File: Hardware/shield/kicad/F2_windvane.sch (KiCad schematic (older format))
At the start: 7 parts, among them U1 MCP6244

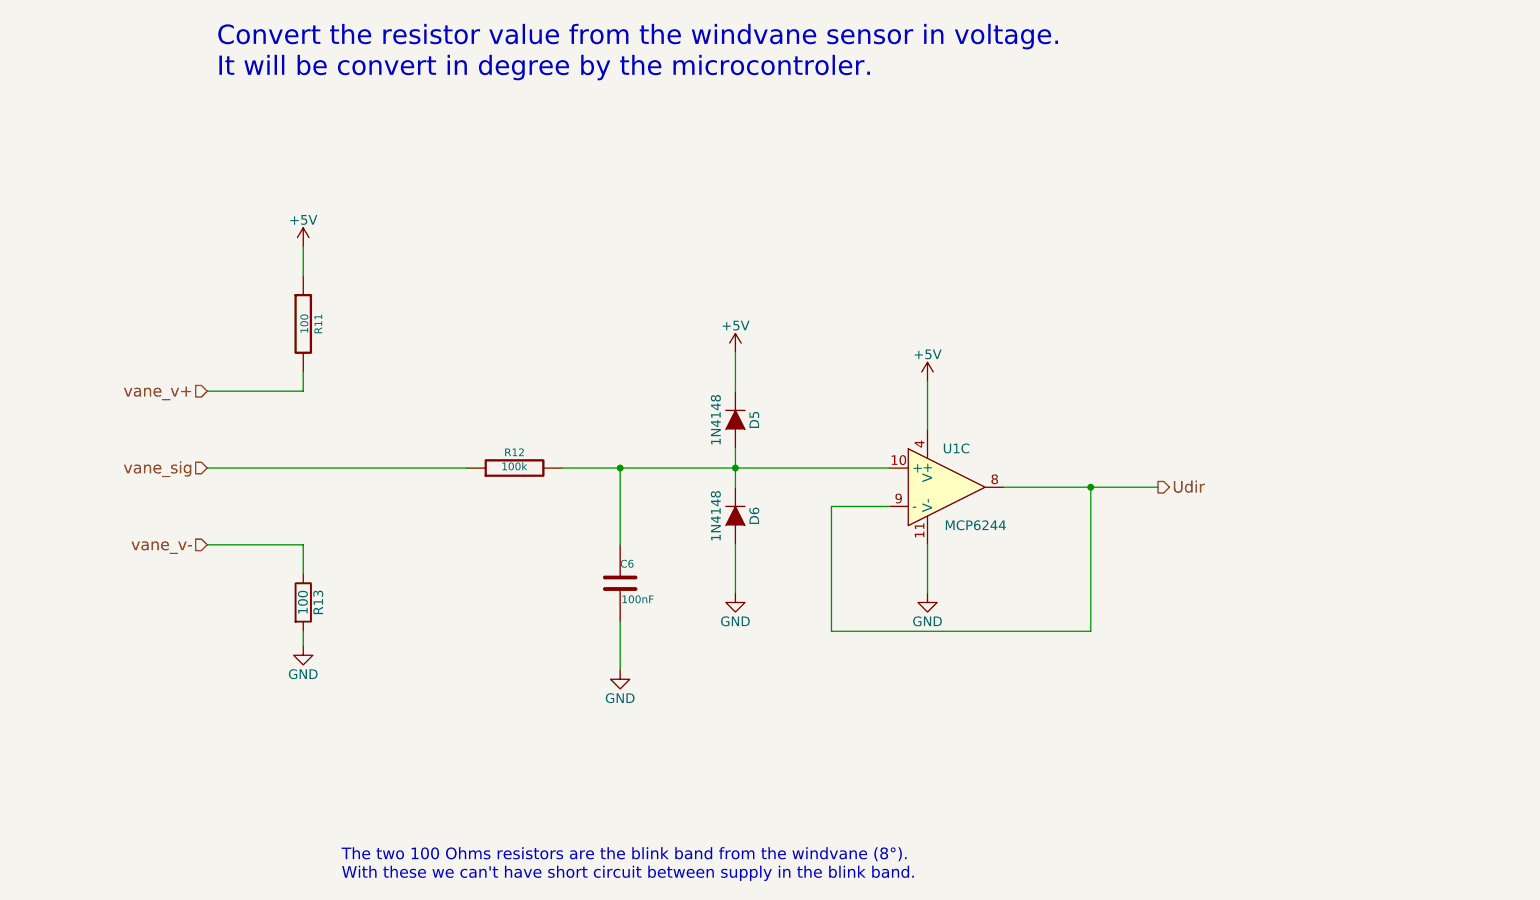
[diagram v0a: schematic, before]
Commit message: move to digital 1.1.1
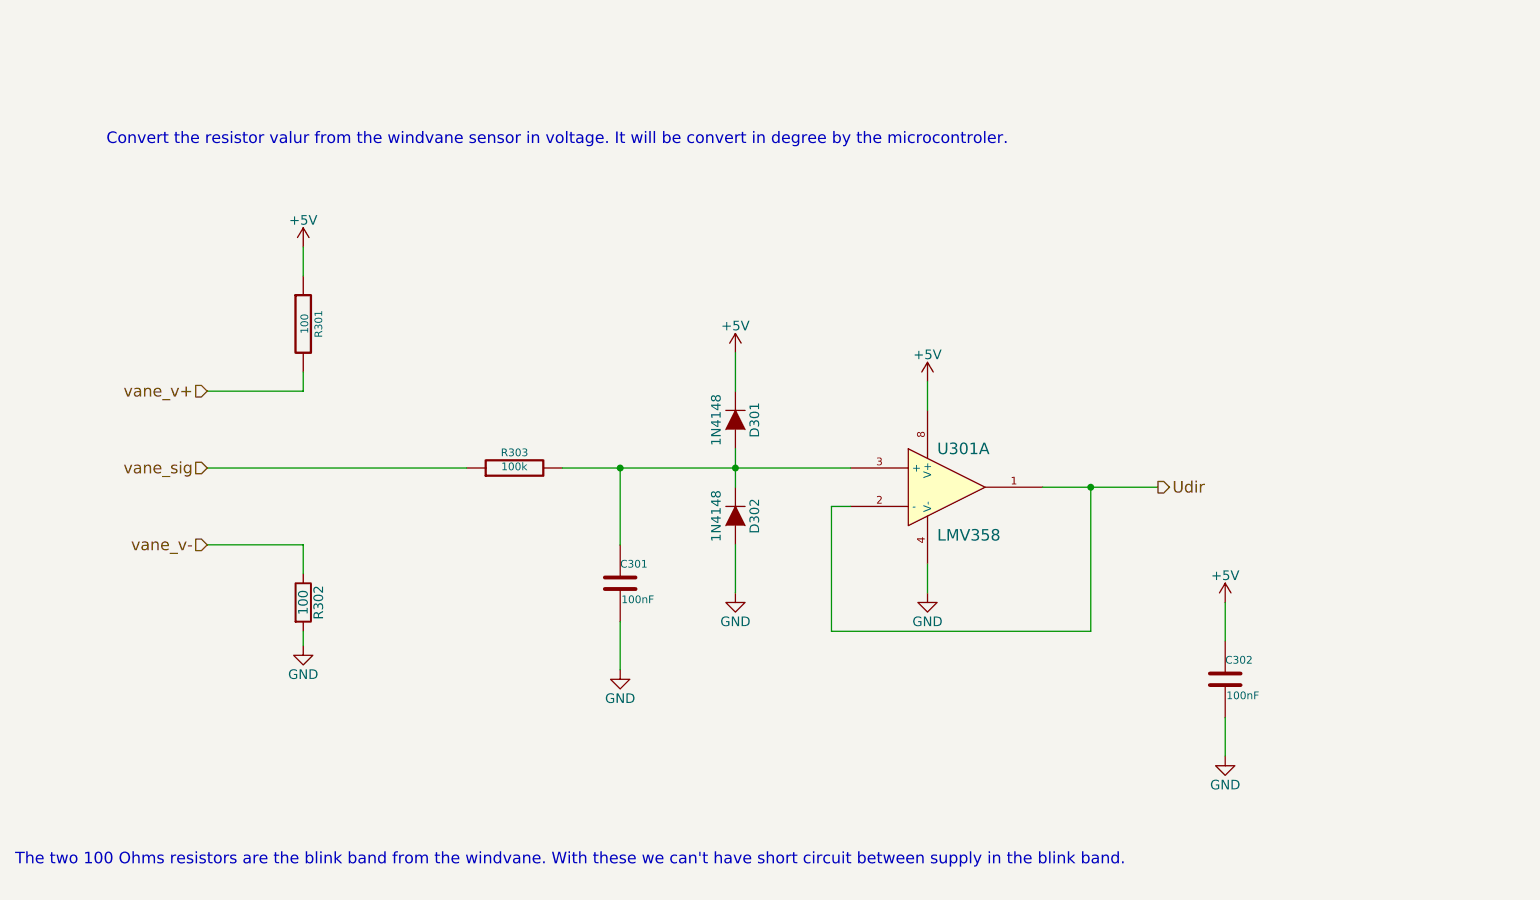
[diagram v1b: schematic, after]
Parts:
- removed U1: MCP6244, Housings_DIP:DIP-14_W7.62mm_LongPads, symbol MCP6004
- added C302: 100nF, Capacitors_ThroughHole:C_Rect_L7_W2.5_P5, symbol C-RESCUE-Windlogger
- added U301: LMV358, Housings_DIP:DIP-8_W7.62mm_LongPads, symbol LM358-RESCUE-Windlogger
- D301: renamed from D5; footprint Discret:DO-35 -> Diodes_ThroughHole:Diode_DO-35_SOD27_Horizontal_RM10
- D302: renamed from D6; footprint Discret:DO-35 -> Diodes_ThroughHole:Diode_DO-35_SOD27_Horizontal_RM10
- R301: renamed from R11; footprint Discret:R3-LARGE_PADS -> Discret:R4
- R302: renamed from R13; footprint Discret:R3-LARGE_PADS -> Discret:R4
- R303: renamed from R12; footprint Discret:R3-LARGE_PADS -> Discret:R4
- renumbered C6 to C301
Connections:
- net +5V: now also C302.1, U301.8 (V+)
- net GND: now also C302.2, U301.4 (V-)
- net Udir: now also U301.1, U301.2 (-)
- net at C301.1, D301.2 (A), D302.1 (K)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: now also U301.3 (+)
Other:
- note added: "Convert the resistor valur from the windvane sensor in voltage. It will be convert in degree by the microcontroler."
- note added: "The two 100 Ohms resistors are the blink band from the windvane. With these we can't have short circuit between supply in the blink band."
- note removed: "Convert the resistor value from the windvane sensor in voltage. \nIt will be convert in degree by the microcontroler."
- note removed: "The two 100 Ohms resistors are the blink band from the windvane (8°).\nWith these we can't have short circuit between supply in the blink band."
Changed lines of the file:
@@
 $Descr A4 11693 8268
 encoding utf-8
-Sheet 3 5
+Sheet 3 6
 Title "Windvane function"
 Date "2016-10-16"
@@
 $EndDescr
 $Comp
-L R-RESCUE-Windlogger R11
+L R-RESCUE-Windlogger R301
 U 1 1 561261A3
 P 4050 2550
-F 0 "R11" V 4130 2550 40  0000 C CNN
+F 0 "R301" V 4130 2550 40  0000 C CNN
 F 1 "100" V 4057 2551 40  0000 C CNN
-F 2 "Discret:R3-LARGE_PADS" V 3980 2550 30  0001 C CNN
+F 2 "Discret:R4" V 3980 2550 30  0001 C CNN
 F 3 "~" H 4050 2550 30  0000 C CNN
 F 4 "0.125W" V 4050 2550 60  0001 C CNN "Puissance"
@@
 $EndComp
 $Comp
-L C-RESCUE-Windlogger C6
+L C-RESCUE-Windlogger C301
 U 1 1 561264FC
 P 5700 3900
-F 0 "C6" H 5700 4000 40  0000 L CNN
+F 0 "C301" H 5700 4000 40  0000 L CNN
 F 1 "100nF" H 5706 3815 40  0000 L CNN
 F 2 "Capacitors_ThroughHole:C_Rect_L7_W2.5_P5" H 5738 3750 30  0001 C CNN
@@
 	4050 2150 4050 2300
 Wire Wire Line
-	7700 3400 8500 3400
+	7900 3400 8500 3400
 Wire Wire Line
 	5700 3300 5700 3700
@@
 	5700 4350 5700 4100
 Wire Wire Line
-	7300 2850 7300 3100
-Wire Wire Line
-	7300 3700 7300 3950
+	7300 3000 7300 2850
+Wire Wire Line
+	7300 3800 7300 3950
 Text HLabel 8500 3400 2    60   Output ~ 0
 Udir
@@
 vane_sig
 $Comp
-L R-RESCUE-Windlogger R12
+L C-RESCUE-Windlogger C302
+U 1 1 56126B37
+P 8850 4400
+F 0 "C302" H 8850 4500 40  0000 L CNN
+F 1 "100nF" H 8856 4315 40  0000 L CNN
+F 2 "Capacitors_ThroughHole:C_Rect_L7_W2.5_P5" H 8888 4250 30  0001 C CNN
+F 3 "~" H 8850 4400 60  0000 C CNN
+F 4 "25V" H 8850 4400 60  0001 C CNN "Tension"
+	1    8850 4400
+	1    0    0    -1
+$EndComp
+Wire Wire Line
+	8850 4000 8850 4200
+Wire Wire Line
+	8850 4600 8850 4800
+$Comp
+L R-RESCUE-Windlogger R303
 U 1 1 5612799B
 P 5150 3300
-F 0 "R12" V 5230 3300 40  0000 C CNN
+F 0 "R303" V 5230 3300 40  0000 C CNN
 F 1 "100k" V 5157 3301 40  0000 C CNN
-F 2 "Discret:R3-LARGE_PADS" V 5080 3300 30  0001 C CNN
+F 2 "Discret:R4" V 5080 3300 30  0001 C CNN
 F 3 "~" H 5150 3300 30  0000 C CNN
 F 4 "0.125W" V 5150 3300 60  0001 C CNN "Puissance"
@@
 	3550 3300 4900 3300
 Wire Wire Line
-	5400 3300 7100 3300
+	5400 3300 6900 3300
 Wire Wire Line
 	8150 4150 8150 3400
@@
 vane_v-
 Wire Wire Line
-	6800 3500 7100 3500
+	6900 3500 6800 3500
 Wire Wire Line
 	6800 3500 6800 4150
@@
 	6300 3700 6300 3950
 $Comp
-L +5V #PWR034
+L LM358-RESCUE-Windlogger U301
+U 1 1 561263BB
+P 7400 3400
+F 0 "U301" H 7350 3600 60  0000 L CNN
+F 1 "LMV358" H 7350 3150 60  0000 L CNN
+F 2 "Housings_DIP:DIP-8_W7.62mm_LongPads" H 7400 3400 60  0001 C CNN
+F 3 "" H 7400 3400 60  0000 C CNN
+	1    7400 3400
+	1    0    0    -1
+$EndComp
+$Comp
+L +5V #PWR031
 U 1 1 573BED92
 P 7300 2850
-F 0 "#PWR034" H 7300 2700 50  0001 C CNN
+F 0 "#PWR031" H 7300 2700 50  0001 C CNN
 F 1 "+5V" H 7300 2990 50  0000 C CNN
 F 2 "" H 7300 2850 50  0000 C CNN
@@
 $EndComp
 $Comp
-L +5V #PWR035
+L +5V #PWR032
+U 1 1 573BEDC7
+P 8850 4000
+F 0 "#PWR032" H 8850 3850 50  0001 C CNN
+F 1 "+5V" H 8850 4140 50  0000 C CNN
+F 2 "" H 8850 4000 50  0000 C CNN
+F 3 "" H 8850 4000 50  0000 C CNN
+	1    8850 4000
+	1    0    0    -1
+$EndComp
+$Comp
+L +5V #PWR033
 U 1 1 573D0C26
 P 4050 2150
-F 0 "#PWR035" H 4050 2000 50  0001 C CNN
+F 0 "#PWR033" H 4050 2000 50  0001 C CNN
 F 1 "+5V" H 4050 2290 50  0000 C CNN
 F 2 "" H 4050 2150 50  0000 C CNN
@@
 $EndComp
 $Comp
-L +5V #PWR036
+L +5V #PWR034
 U 1 1 573D0D74
 P 6300 2700
-F 0 "#PWR036" H 6300 2550 50  0001 C CNN
+F 0 "#PWR034" H 6300 2550 50  0001 C CNN
 F 1 "+5V" H 6300 2840 50  0000 C CNN
 F 2 "" H 6300 2700 50  0000 C CNN
@@
 $EndComp
 $Comp
-L R R13
+L R R302
 U 1 1 57E81F25
 P 4050 4000
-F 0 "R13" V 4130 4000 50  0000 C CNN
+F 0 "R302" V 4130 4000 50  0000 C CNN
 F 1 "100" V 4050 4000 50  0000 C CNN
-F 2 "Discret:R3-LARGE_PADS" V 3980 4000 50  0001 C CNN
+F 2 "Discret:R4" V 3980 4000 50  0001 C CNN
 F 3 "" H 4050 4000 50  0000 C CNN
 	1    4050 4000
@@
 Wire Wire Line
 	4050 4150 4050 4150
-Text Notes 3600 1275 0    100  ~ 0
-Convert the resistor value from the windvane sensor in voltage. \nIt will be convert in degree by the microcontroler.
-Text Notes 4250 5450 0    60   ~ 0
-The two 100 Ohms resistors are the blink band from the windvane (8°).\nWith these we can't have short circuit between supply in the blink band.
-$Comp
-L GND #PWR037
+Text Notes 3025 1625 0    60   ~ 0
+Convert the resistor valur from the windvane sensor in voltage. It will be convert in degree by the microcontroler.
+Text Notes 2550 5375 0    60   ~ 0
+The two 100 Ohms resistors are the blink band from the windvane. With these we can't have short circuit between supply in the blink band.
+$Comp
+L GND #PWR035
 U 1 1 58046061
 P 4050 4225
-F 0 "#PWR037" H 4050 3975 50  0001 C CNN
+F 0 "#PWR035" H 4050 3975 50  0001 C CNN
 F 1 "GND" H 4050 4075 50  0000 C CNN
 F 2 "" H 4050 4225 50  0000 C CNN
@@
 	4050 4225 4050 4150
 $Comp
-L GND #PWR038
+L GND #PWR036
 U 1 1 580460B8
 P 5700 4350
-F 0 "#PWR038" H 5700 4100 50  0001 C CNN
+F 0 "#PWR036" H 5700 4100 50  0001 C CNN
 F 1 "GND" H 5700 4200 50  0000 C CNN
 F 2 "" H 5700 4350 50  0000 C CNN
@@
 $EndComp
 $Comp
-L GND #PWR039
+L GND #PWR037
 U 1 1 580460EC
 P 6300 3950
-F 0 "#PWR039" H 6300 3700 50  0001 C CNN
+F 0 "#PWR037" H 6300 3700 50  0001 C CNN
 F 1 "GND" H 6300 3800 50  0000 C CNN
 F 2 "" H 6300 3950 50  0000 C CNN
@@
 $EndComp
 $Comp
-L GND #PWR040
+L GND #PWR038
 U 1 1 58046118
 P 7300 3950
-F 0 "#PWR040" H 7300 3700 50  0001 C CNN
+F 0 "#PWR038" H 7300 3700 50  0001 C CNN
 F 1 "GND" H 7300 3800 50  0000 C CNN
 F 2 "" H 7300 3950 50  0000 C CNN
@@
 $EndComp
 $Comp
-L D D5
+L GND #PWR039
+U 1 1 58046144
+P 8850 4800
+F 0 "#PWR039" H 8850 4550 50  0001 C CNN
+F 1 "GND" H 8850 4650 50  0000 C CNN
+F 2 "" H 8850 4800 50  0000 C CNN
+F 3 "" H 8850 4800 50  0000 C CNN
+	1    8850 4800
+	1    0    0    -1
+$EndComp
+$Comp
+L D D301
 U 1 1 580461AD
 P 6300 3050
-F 0 "D5" H 6300 3150 50  0000 C CNN
+F 0 "D301" H 6300 3150 50  0000 C CNN
 F 1 "1N4148" H 6300 2950 50  0000 C CNN
-F 2 "Discret:DO-35" H 6300 3050 50  0001 C CNN
+F 2 "Diodes_ThroughHole:Diode_DO-35_SOD27_Horizontal_RM10" H 6300 3050 50  0001 C CNN
 F 3 "" H 6300 3050 50  0000 C CNN
 	1    6300 3050
@@
 $EndComp
 $Comp
-L D D6
+L D D302
 U 1 1 58046207
 P 6300 3550
-F 0 "D6" H 6300 3650 50  0000 C CNN
+F 0 "D302" H 6300 3650 50  0000 C CNN
 F 1 "1N4148" H 6300 3450 50  0000 C CNN
-F 2 "Discret:DO-35" H 6300 3550 50  0001 C CNN
+F 2 "Diodes_ThroughHole:Diode_DO-35_SOD27_Horizontal_RM10" H 6300 3550 50  0001 C CNN
 F 3 "" H 6300 3550 50  0000 C CNN
 	1    6300 3550
 	0    1    1    0
 $EndComp
-$Comp
-L MCP6004 U1
-U 3 1 58593AA6
-P 7400 3400
-F 0 "U1" H 7450 3600 50  0000 C CNN
-F 1 "MCP6244" H 7550 3200 50  0000 C CNN
-F 2 "Housings_DIP:DIP-14_W7.62mm_LongPads" H 7350 3500 50  0001 C CNN
-F 3 "" H 7450 3600 50  0000 C CNN
-	3    7400 3400
-	1    0    0    -1
-$EndComp
 $EndSCHEMATC
